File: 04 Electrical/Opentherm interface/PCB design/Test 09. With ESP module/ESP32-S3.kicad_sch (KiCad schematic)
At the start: 5 parts, among them U1 ESP32-S3-WROOM-1-N8R2

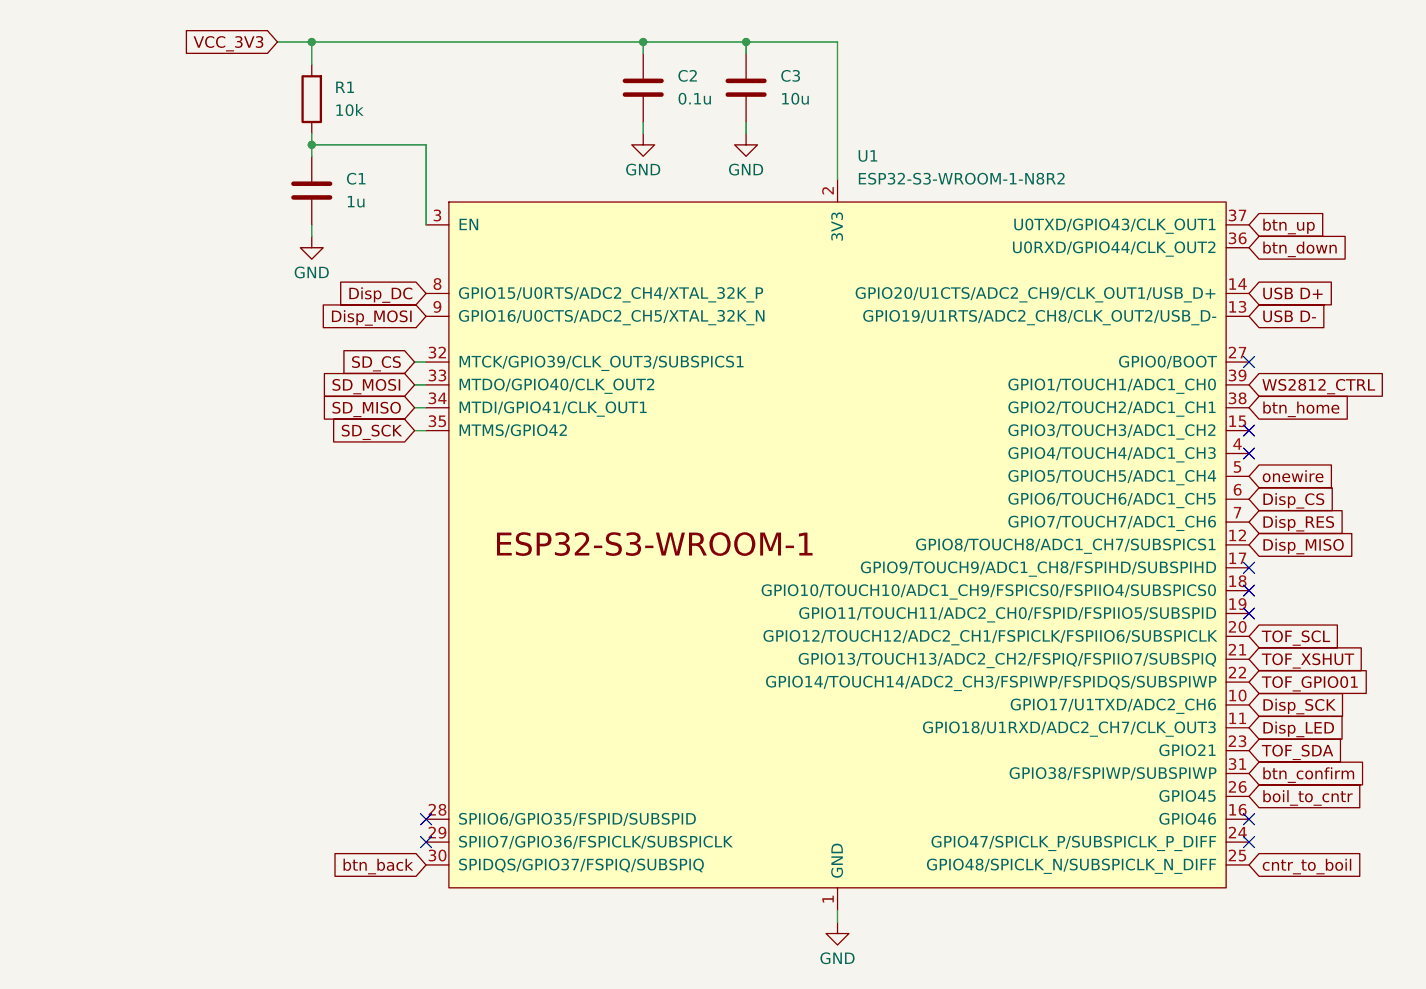
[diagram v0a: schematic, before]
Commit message: Schematic update
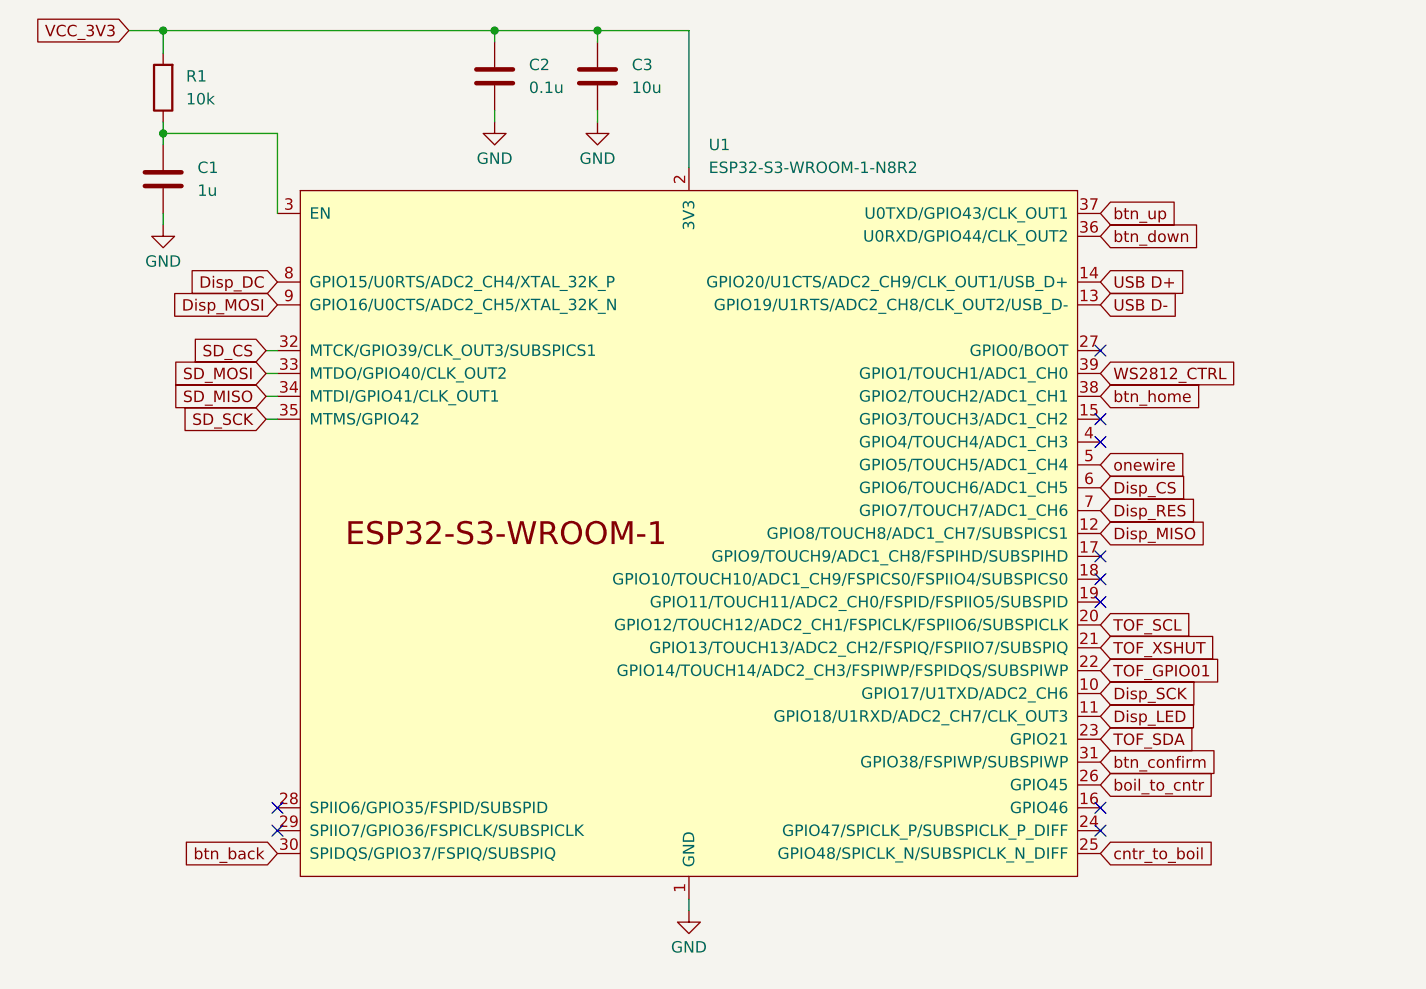
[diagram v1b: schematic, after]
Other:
- moved on the sheet: C1, C2, C3, R1, U1
